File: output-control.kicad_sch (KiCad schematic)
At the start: 57 parts, among them U17 ADS7828, U18 TCA9534PWR, U19 ADS7828

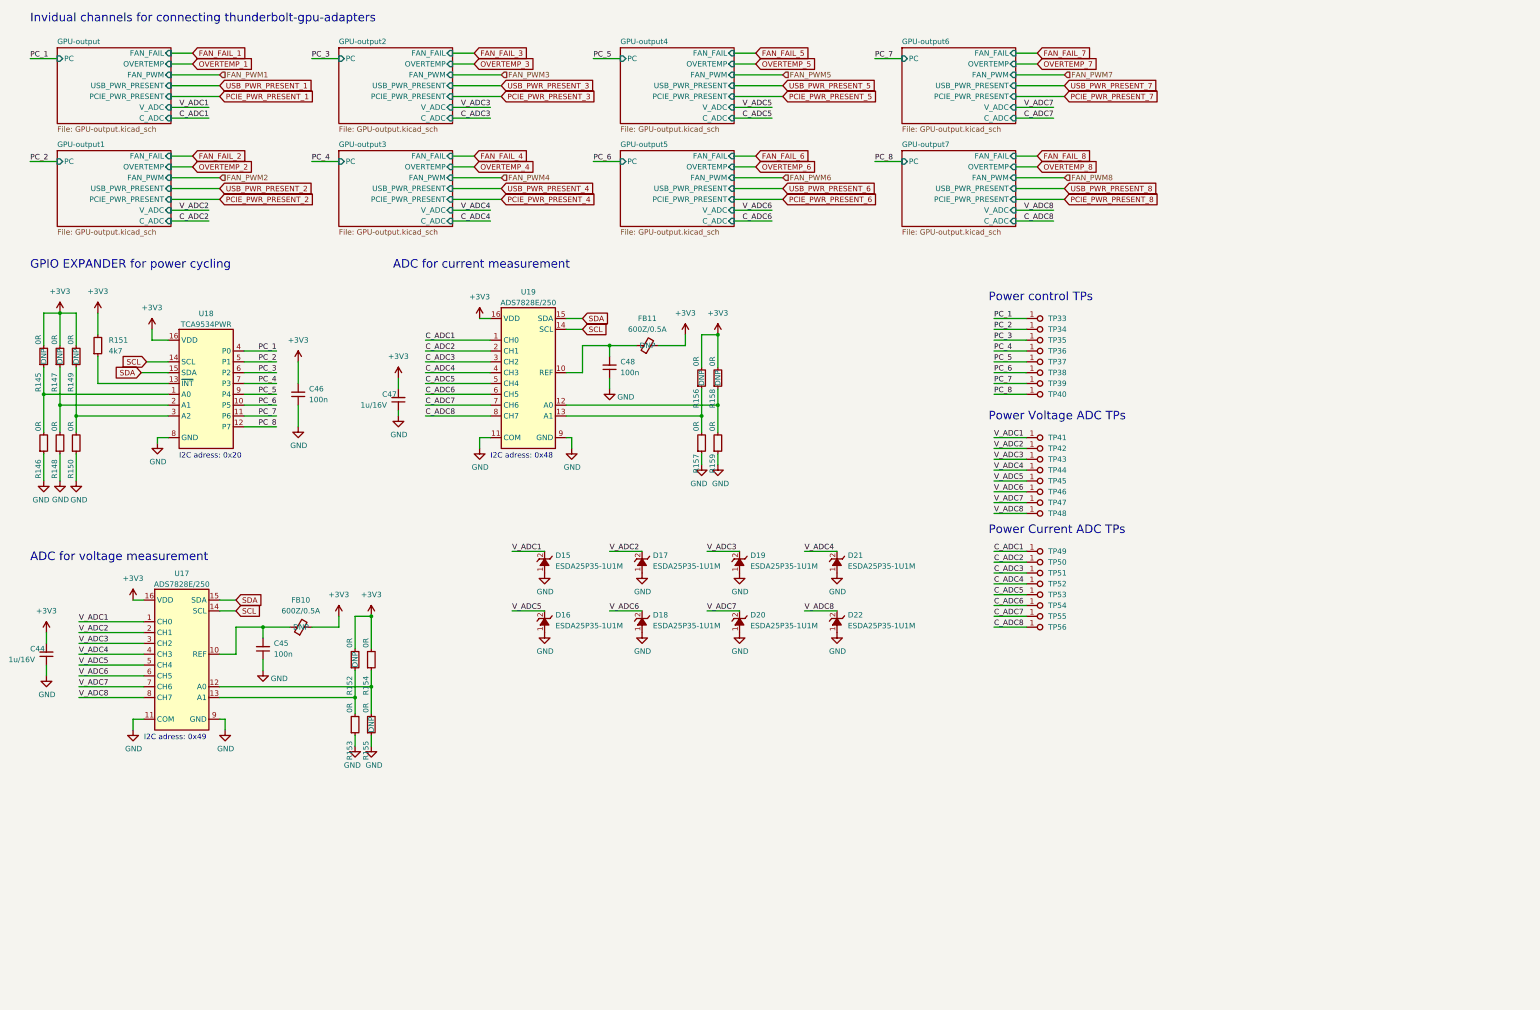
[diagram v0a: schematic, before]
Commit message: Additional cleanup
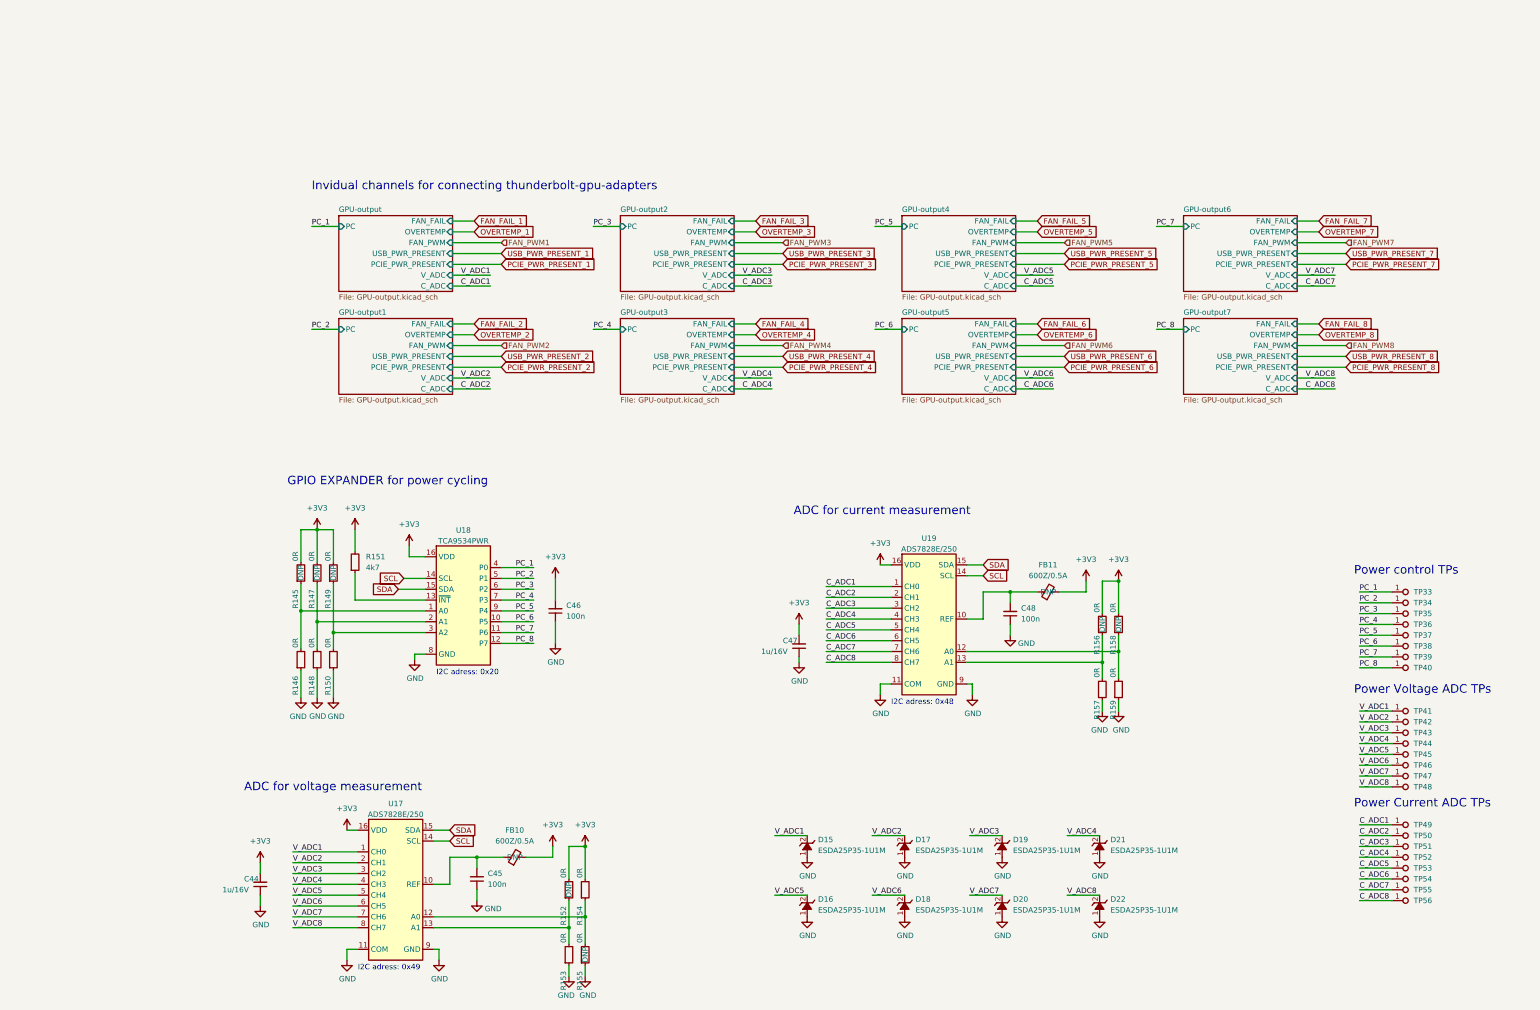
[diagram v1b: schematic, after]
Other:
- title: (none) -> GPU Cluster Backplane
- moved on the sheet: C44, C45, C46, C47, C48, D15, D16, D17, D18, D19, D20, D21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
